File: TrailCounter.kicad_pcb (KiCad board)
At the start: 2 copper layers, 173.9 x 114.5 mm, 59 parts, among them IC1 BQ24032ARHLR, IC2 AP9211SA-AD-HAC-7, IC3 MAX20404AFOD_VY+, IC4 PIC32CM5164LE00048-I_Y8X, IC5 NVT2002DP,118, IC6 NVT2002DP,118, J1 Micro USB, J2 SD_CARD, J3 RTC, J4 PIR, J5 PROGRAMMING, Q1 PMN16XNEX, Q2 PMN16XNEX, U1 12BHC186P-GR, U2 12BHC186P-GR, U3 TPS61230ARNSR, U4 WirelesStickV3, U5 CoralMicro

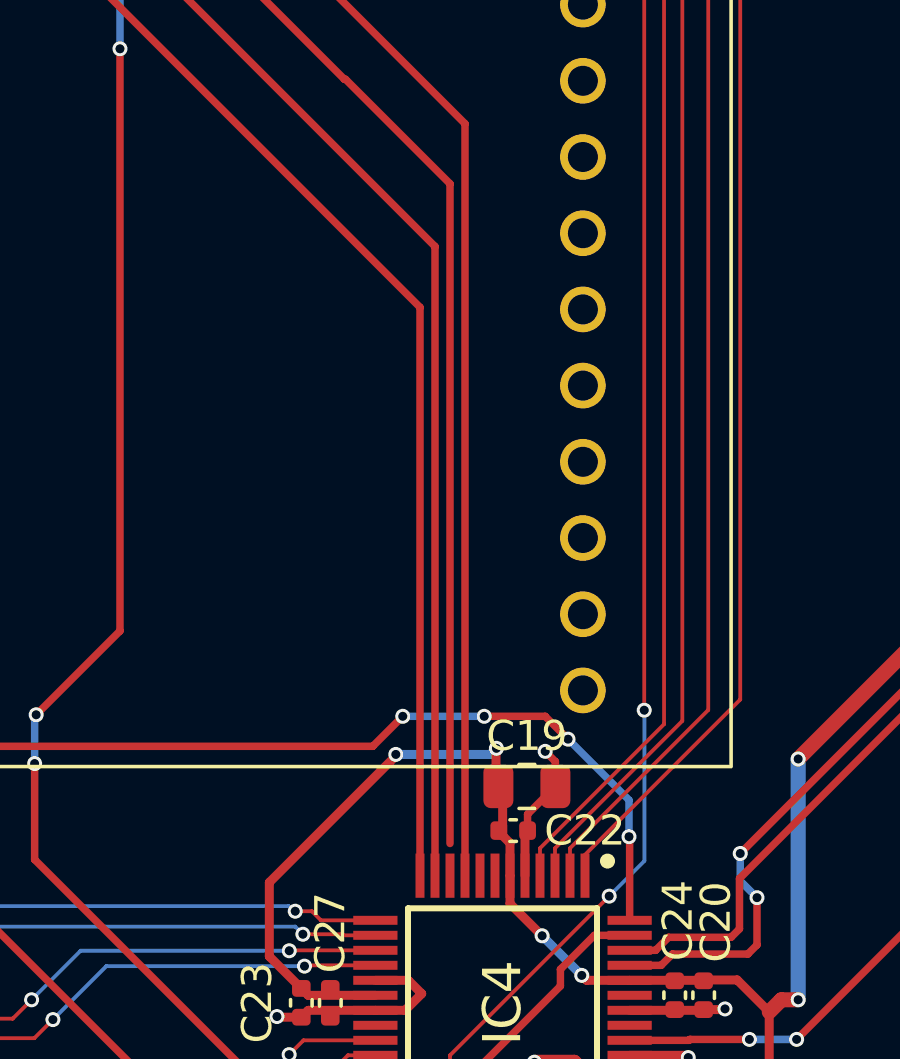
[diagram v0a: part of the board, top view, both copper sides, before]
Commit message: changes
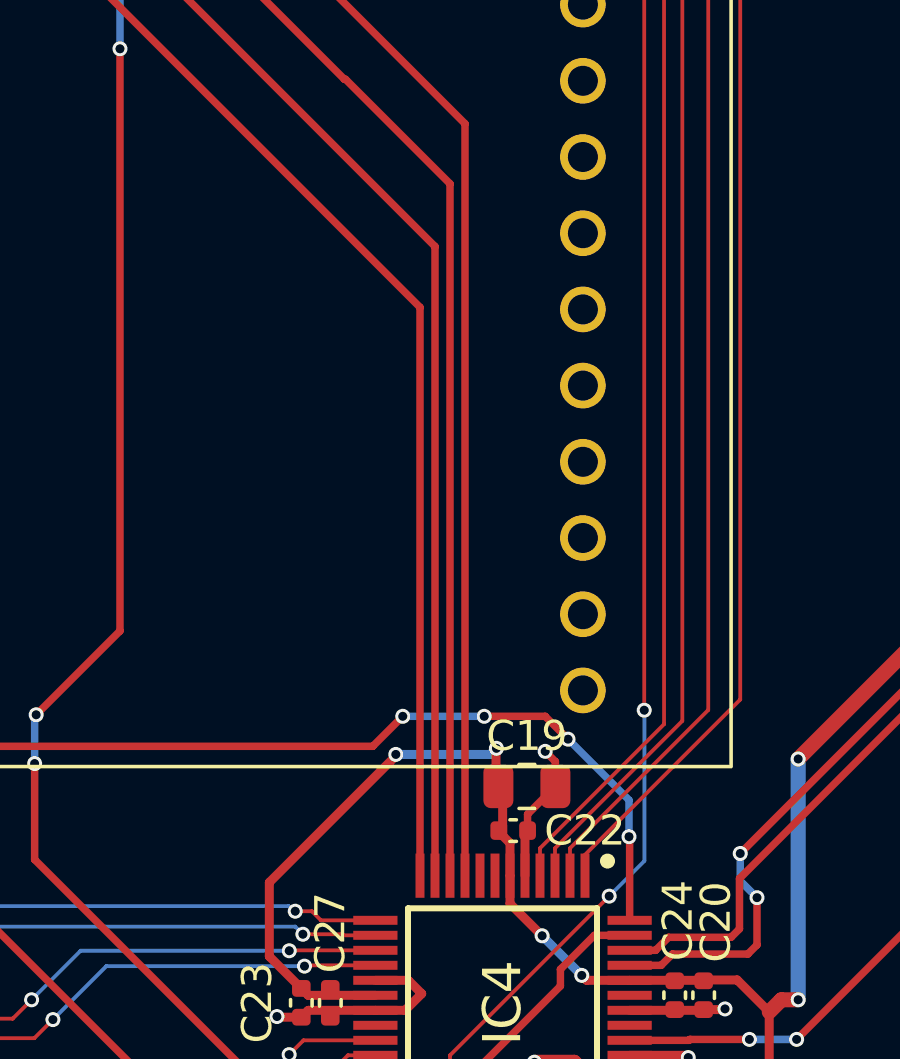
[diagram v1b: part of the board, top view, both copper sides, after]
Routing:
- net /SCK_2: track 44.8 -> 45.9 mm
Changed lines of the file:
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@@
   (segment (start 168.676 63.66) (end 168.676 88.726) (width 0.25) (layer "F.Cu") (net 37))
   (segment (start 152.006 46.99) (end 168.676 63.66) (width 0.25) (layer "F.Cu") (net 37))
+  (segment (start 168.176 65.6616) (end 168.176 88.726) (width 0.25) (layer "F.Cu") (net 38))
   (segment (start 164.6936 62.1792) (end 168.176 65.6616) (width 0.25) (layer "F.Cu") (net 38))
-  (segment (start 168.176 65.6616) (end 168.176 87.6528) (width 0.25) (layer "F.Cu") (net 38))
+  (segment (start 152.006 49.53) (end 164.6552 62.1792) (width 0.25) (layer "F.Cu") (net 38))
   (segment (start 164.6552 62.1792) (end 164.6936 62.1792) (width 0.25) (layer "F.Cu") (net 38))
-  (segment (start 152.006 49.53) (end 164.6552 62.1792) (width 0.25) (layer "F.Cu") (net 38))
   (segment (start 152.006 52.07) (end 158.242 58.306) (width 0.25) (layer "F.Cu") (net 39))
   (segment (start 158.242 58.306) (end 158.242 58.3184) (width 0.25) (layer "F.Cu") (net 39))
